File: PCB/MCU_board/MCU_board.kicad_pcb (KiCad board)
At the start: 4 copper layers, 70 x 70 mm, 46 parts, among them IC1 NEO-F10N-00B, IC2 TXB0104PWR, IC3 ESP32-S3-WROOM-1-N4R8, IC6 4259-63, IC8 MAX98357AETE+T, J1 DS1013-40SSIB1-B-0, J4 FXP612 (u.FL) 2, J5 FXP612 (u.FL) 1, J6 SIM8055-6-1-14-00-A, J7 FXP612 (u.FL) 1, Q3 Si2323DDS-T1-GE3, Q5 BSS138, U2 SIM7000G

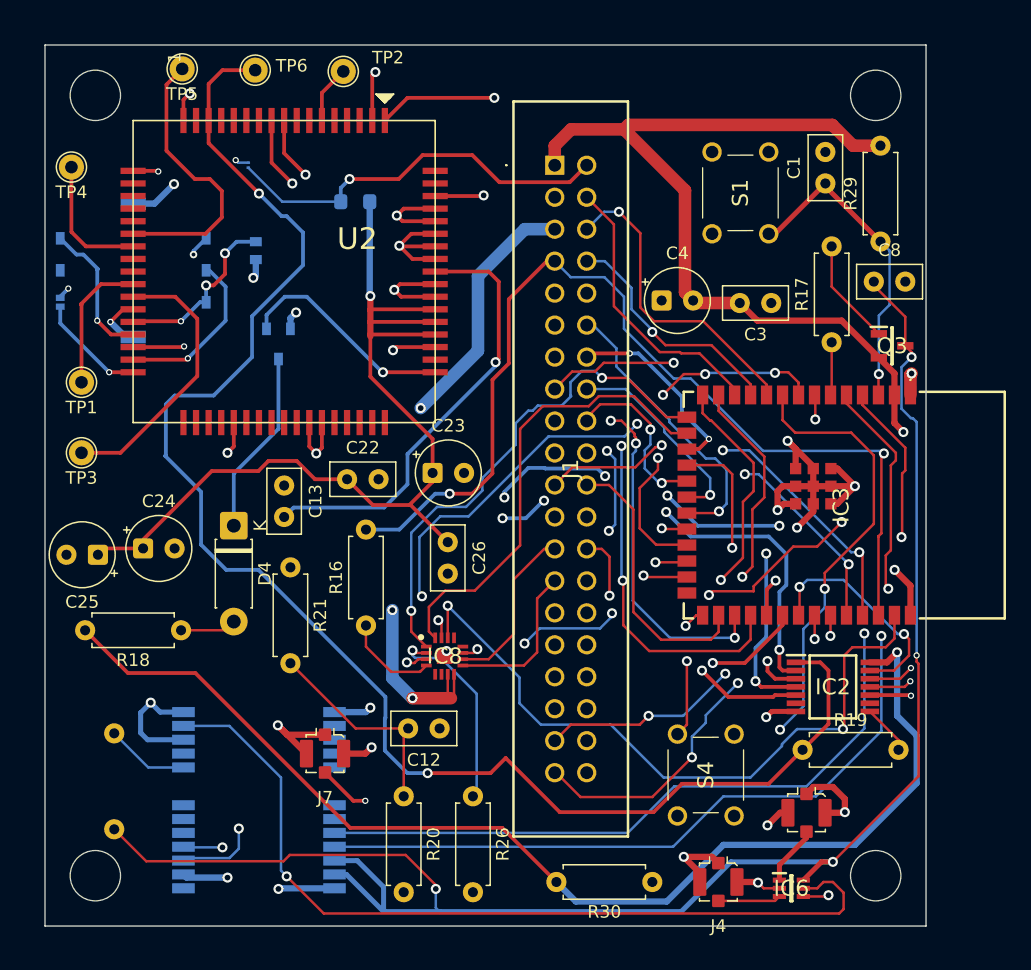
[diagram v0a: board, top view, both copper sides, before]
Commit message: everything checked
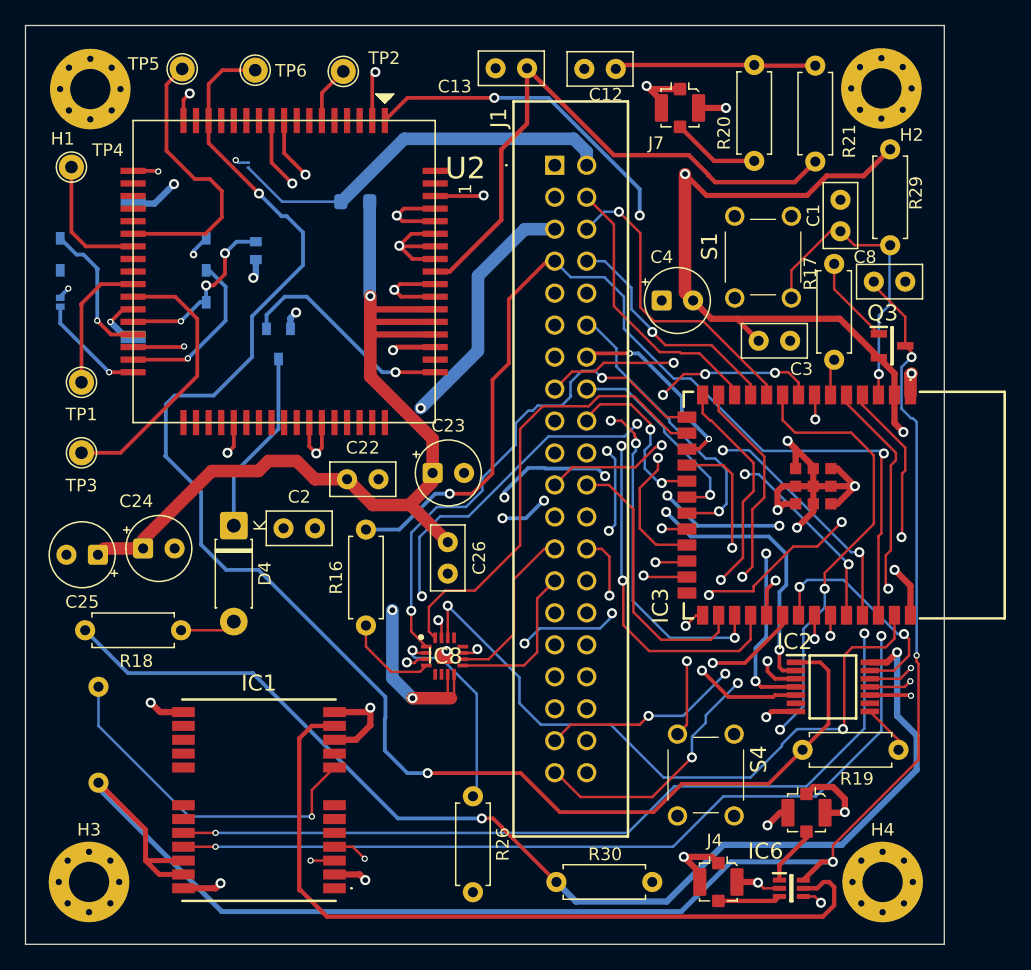
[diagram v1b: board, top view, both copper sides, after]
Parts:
- added C2: 100nF, Capacitor_THT:C_Disc_D5.0mm_W2.5mm_P2.50mm, F.Cu at (49.0, 138.4)
- added H1: MountingHole, MountingHole:MountingHole_3.2mm_M3_Pad_Via, F.Cu at (33.6, 103.5)
- added H2: MountingHole, MountingHole:MountingHole_3.2mm_M3_Pad_Via, F.Cu at (96.5, 103.5)
- added H3: MountingHole, MountingHole:MountingHole_3.2mm_M3_Pad_Via, F.Cu at (33.5, 166.5)
- added H4: MountingHole, MountingHole:MountingHole_3.2mm_M3_Pad_Via, F.Cu at (96.5, 166.5)
- IC1: moved to F.Cu
- moved R20 64.4 mm to (86.3, 101.6)
- moved J7 58.5 mm to (80.5, 105.0)
- moved C12 53.6 mm to (72.8, 101.9), turned to 0 degrees
- moved R21 52.7 mm to (91.2, 109.3), turned to 90 degrees
- moved C13 37.2 mm to (65.8, 101.8), turned to 0 degrees
- moved S1 5.41 mm to (84.8, 120.1)
- moved C1 3.98 mm to (93.2, 114.8)
- moved R28 3.91 mm to (34.2, 158.6)
- moved C3 3.35 mm to (89.2, 123.5)
- moved R17 1.40 mm to (92.7, 125.0)
- moved R29 0.82 mm to (97.2, 115.9)
- turned IC1 to 0 degrees
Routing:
- net /Stationary/GSM_sheet/SIM_POWER: track 14.1 -> 37.0 mm
- net Net-(IC1-RESET_N): track 6.62 -> 27.7 mm, vias 0 -> 1
- net /TXD: track 76.4 -> 88.4 mm, vias 2 -> 3
- net /RXD: track 74.9 -> 86.9 mm, vias 2 -> 3
- net Net-(U2-RF_ANT): track 39.6 -> 47.2 mm, vias 1 -> 0
- net /GSM_INT: track 77.4 -> 70.5 mm
- net GND: track 142.0 -> 135.6 mm
- net Net-(J7-In): track 12.7 -> 7.02 mm, vias 1 -> 0
- net Net-(IC1-RF_IN): track 68.2 -> 63.3 mm, vias 1 -> 0
- net /TIMEPULSE: track 73.9 -> 76.2 mm
- net /+3V3: track 179.2 -> 181.3 mm, vias 2 -> 4
- net /Stationary/GSM_sheet/PWRKEY_1V8: track 72.6 -> 71.1 mm, vias 3 -> 4
- net Net-(Q3-G): track 8.50 -> 7.31 mm
- net /GSM_POWER: track 4.22 -> 3.04 mm
- net Net-(C12-Pad2): track 17.0 -> 16.0 mm
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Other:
- board size 70 x 70 mm -> 73 x 73 mm
